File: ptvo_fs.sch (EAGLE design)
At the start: 30 parts, among them IC1 DS18S20USOP8, U1 HTU21D

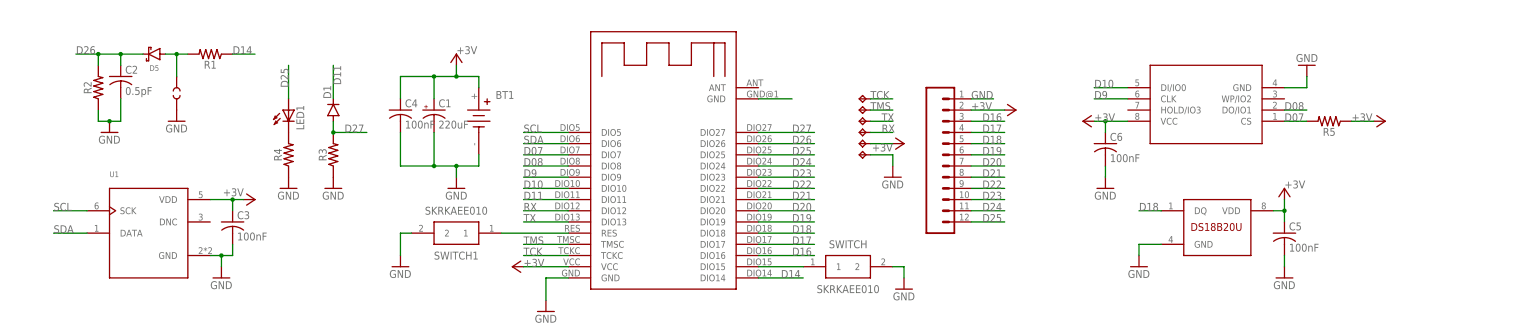
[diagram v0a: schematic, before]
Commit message: Add files via upload
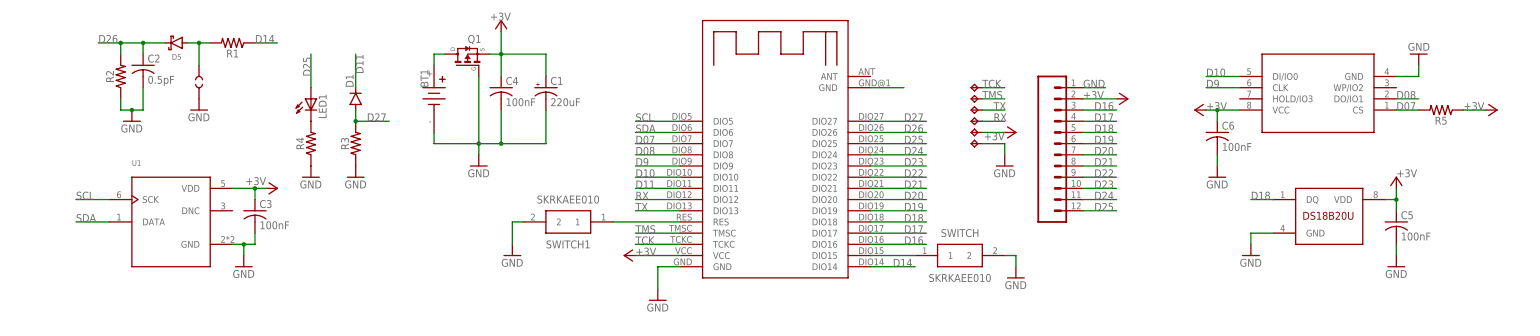
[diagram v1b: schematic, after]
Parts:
- added Q1: SI2323DS, SI2323DS:SI2323DS
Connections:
- new net N$5: BT1.+, Q1.D
- net +3V3: now also Q1.S; no longer BT1.+
- net GND: now also Q1.G
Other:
- moved on the sheet: BT1, C1, C2, C3, C4, C5, C6, D1, D5, LED1, R1, R2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

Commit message: Add files via upload
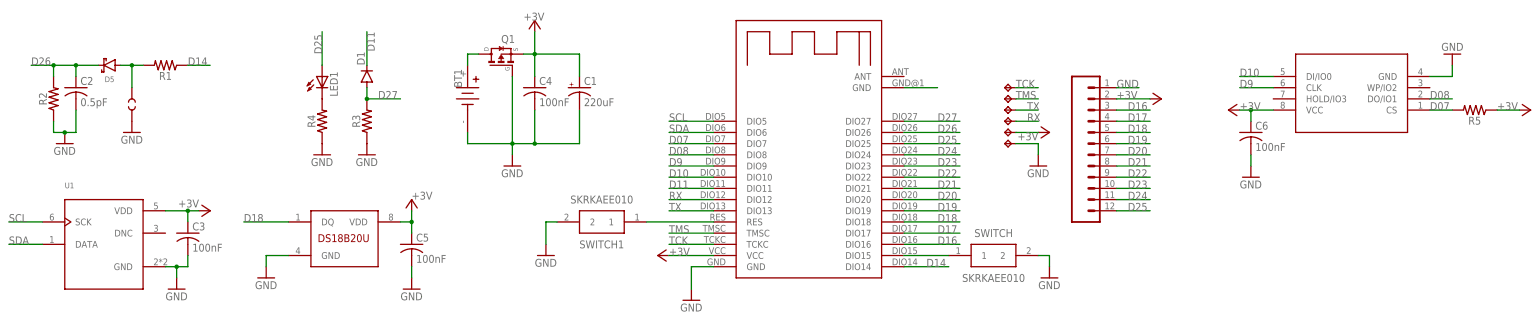
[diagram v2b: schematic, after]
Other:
- moved on the sheet: BT1, C1, C2, C3, C4, C5, C6, D1, D5, LED1, Q1, R1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
